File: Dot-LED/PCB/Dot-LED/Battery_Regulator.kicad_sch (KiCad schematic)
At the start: 1 part, among them IC2 MCP73831T-2ACI_OT

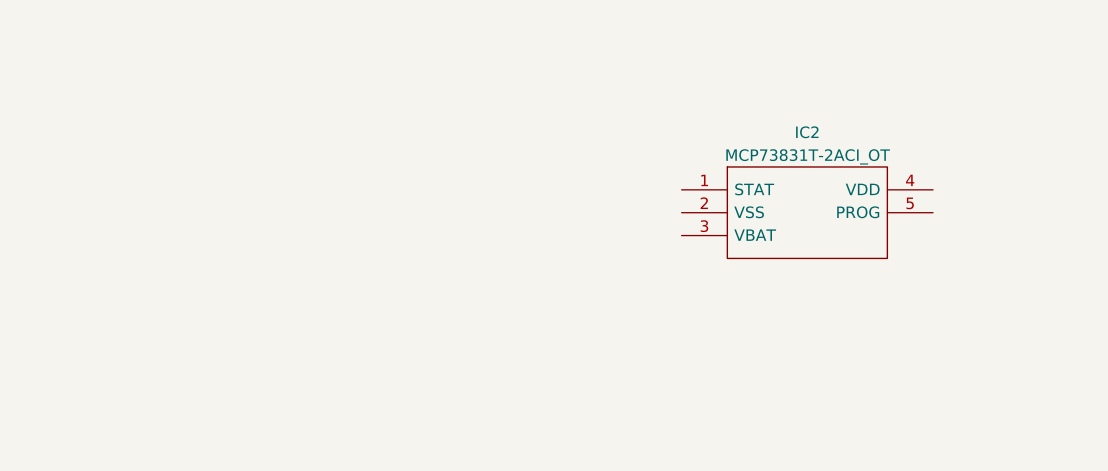
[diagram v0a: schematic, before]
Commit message: Update DotLED Schem
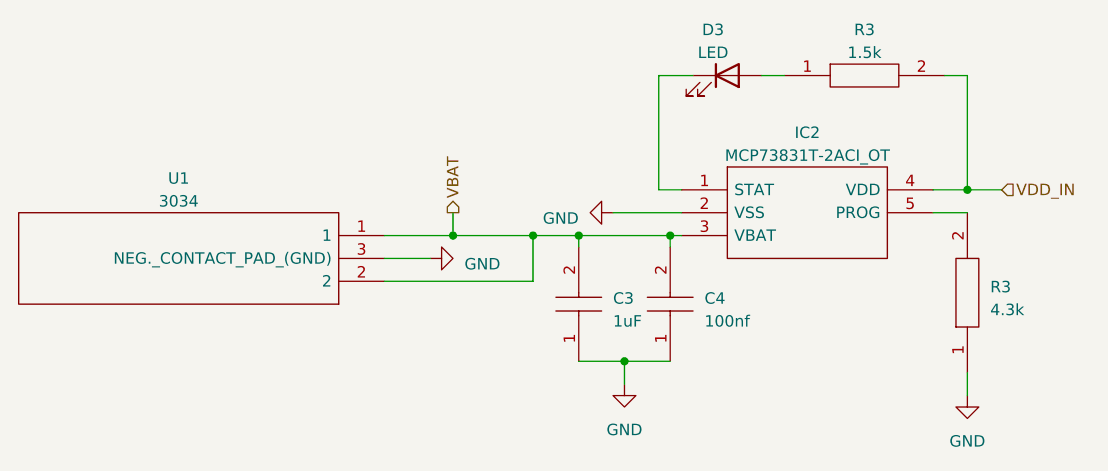
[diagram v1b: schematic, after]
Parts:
- added C3: 1uF, Capacitor_SMD:C_0603_1608Metric_Pad1.08x0.95mm_HandSolder, symbol SamacSys_Parts:0402B102K500NT
- added C4: 100nf, Capacitor_SMD:C_0603_1608Metric_Pad1.08x0.95mm_HandSolder, symbol SamacSys_Parts:0402B102K500NT
- added D3: LED, LED_SMD:LED_0603_1608Metric_Pad1.05x0.95mm_HandSolder, symbol Device:LED
- added R3: 4.3k, RESC1608X55N, symbol SamacSys_Parts:RMCF0603ZT0R00
- added R3: 1.5k, RESC1608X55N, symbol SamacSys_Parts:RMCF0603ZT0R00
- added U1: 3034, 3034, symbol SamacSys_Parts:3034
- IC2: Digi-Key_PN (none) -> 579-MCP73831T-2ACIOT
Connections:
- net at IC2.1 (STAT): now also D3.1 (K)
- net GND: now reaches IC2.2 (VSS)
- net GND: now also C3.1, C4.1, R3.1, U1.3 (NEG._CONTACT_PAD_(GND))
- net VBAT: now reaches IC2.3 (VBAT)
- net VBAT: now also C3.2, C4.2, U1.1, U1.2
- net VDD_IN: now reaches IC2.4 (VDD)
- net VDD_IN: now also R3.2
- net at IC2.5 (PROG): now also R3.2
- new net: D3.2 (A), R3.1
